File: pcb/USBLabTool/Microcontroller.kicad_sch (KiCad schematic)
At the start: 27 parts, among them J1 Conn_01x06_Pin, J2 Conn_02x12_Odd_Even, SW1 TS02-66-73-BK-100-SCR-D, U12 STM32H562VGTx, Y1 32.768kHz, Y2 NX2016SA-25M-EXS00A-CS08742

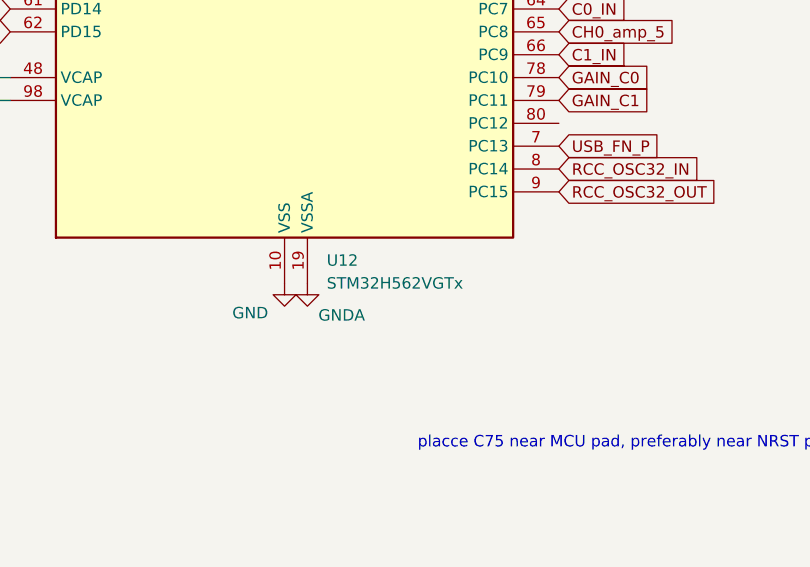
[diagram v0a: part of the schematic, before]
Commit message: try to do logic analyzer
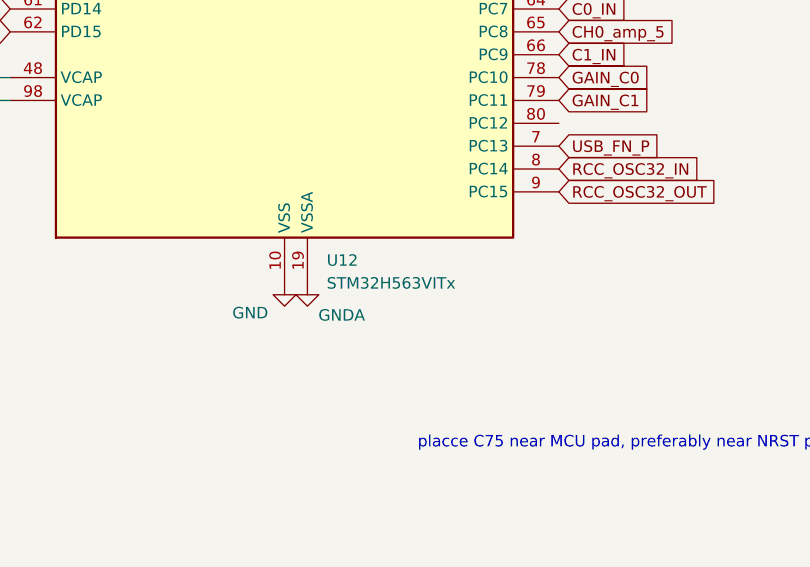
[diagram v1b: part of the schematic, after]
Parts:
- removed U12: STM32H562VGTx, Package_QFP:LQFP-100_14x14mm_P0.5mm, symbol MCU_ST_STM32H5:STM32H562VGTx
- added U12: STM32H563VITx, Package_QFP:LQFP-100_14x14mm_P0.5mm, symbol MCU_ST_STM32H5:STM32H563VITx
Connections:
- net +3.3V: now also U12.100 (VDD), U12.11 (VDD), U12.28 (VDD), U12.50 (VDD), U12.6 (VBAT), U12.73 (VDDUSB), U12.75 (VDD)
- net ADC1_INP0: now also U12.23 (PA0)
- net ADC2_INP3: now also U12.31 (PA6)
- net C0_IN: now also U12.64 (PC7)
- net C1_IN: now also U12.66 (PC9)
- net CH0_ACDC: now also U12.34 (PC5)
- net CH0_amp_1: now also U12.51 (PB12)
- net CH0_amp_10: now also U12.54 (PB15)
- net CH0_amp_2.5: now also U12.63 (PC6)
- net CH0_amp_5: now also U12.65 (PC8)
- net CH0_attenuate: now also U12.52 (PB13)
- net CH1_ACDC: now also U12.33 (PC4)
- net CH1_amp_1: now also U12.35 (PB0)
- net CH1_amp_10: now also U12.47 (PB10)
- net CH1_amp_2.5: now also U12.37 (PB2)
- net CH1_amp_5: now also U12.36 (PB1)
- net CH1_attenuate: now also U12.53 (PB14)
- net DEBUG_JTCK_SWCLK: now also U12.76 (PA14(JTCK)
- net DEBUG_JTD-SW0: now also U12.89 (PB3(JTDO)
- net DEBUG_JTMS-SWDI0: now also U12.72 (PA13(JTMS)
- net GAIN_C0: now also U12.78 (PC10)
- net GAIN_C1: now also U12.79 (PC11)
- net GND: now also U12.10 (VSS), U12.27 (VSS), U12.49 (VSS), U12.74 (VSS), U12.99 (VSS)
- net GNDA: now also U12.19 (VSSA), U12.20 (VREF-)
- net LOGIC_IN0: now also U12.81 (PD0)
- net LOGIC_IN1: now also U12.82 (PD1)
- net LOGIC_IN10: now also U12.60 (PD13)
- net LOGIC_IN11: now also U12.59 (PD12)
- net LOGIC_IN12: now also U12.58 (PD11)
- net LOGIC_IN13: now also U12.57 (PD10)
- net LOGIC_IN14: now also U12.56 (PD9)
- net LOGIC_IN15: now also U12.55 (PD8)
- net LOGIC_IN2: now also U12.83 (PD2)
- net LOGIC_IN3: now also U12.84 (PD3)
- net LOGIC_IN4: now also U12.85 (PD4)
- net LOGIC_IN5: now also U12.86 (PD5)
- net LOGIC_IN6: now also U12.87 (PD6)
- net LOGIC_IN7: now also U12.88 (PD7)
- net LOGIC_IN8: now also U12.62 (PD15)
- net LOGIC_IN9: now also U12.61 (PD14)
- net NRST: now also U12.14 (NRST)
- net RCC_OSC32_IN: now also U12.8 (PC14)
- net RCC_OSC32_OUT: now also U12.9 (PC15)
- net RCC_OSC_IN: now also U12.12 (PH0)
- net RCC_OSC_OUT: now also U12.13 (PH1)
- net TIM1_CH1: now also U12.67 (PA8)
- net TIM1_CH2: now also U12.69 (PA10)
- net TIM2_CH2: now also U12.24 (PA1)
- net TIM2_CH3: now also U12.25 (PA2)
- net UCPD_CC1: now also U12.2 (PE3)
- net UCPD_CC2: now also U12.1 (PE2)
- net UCPD_FLT: now also U12.4 (PE5)
- net USB_FN_N: now also U12.5 (PE6)
- net USB_FN_P: now also U12.7 (PC13)
- net USCPD_DBn: now also U12.3 (PE4)
- net VREFP: now also U12.21 (VREF+)
- net at C31.1, C32.1: now also U12.98 (VCAP)
- net at C31.2, C32.2: now also U12.48 (VCAP)
- net at R54.2, R55.2: now also U12.22 (VDDA)
- net at R53.2: now also U12.94 (BOOT0)
